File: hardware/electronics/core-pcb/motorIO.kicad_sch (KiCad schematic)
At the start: 3 parts, among them J5 1-84952-1, J6 1-84952-1, J7 1-84952-1

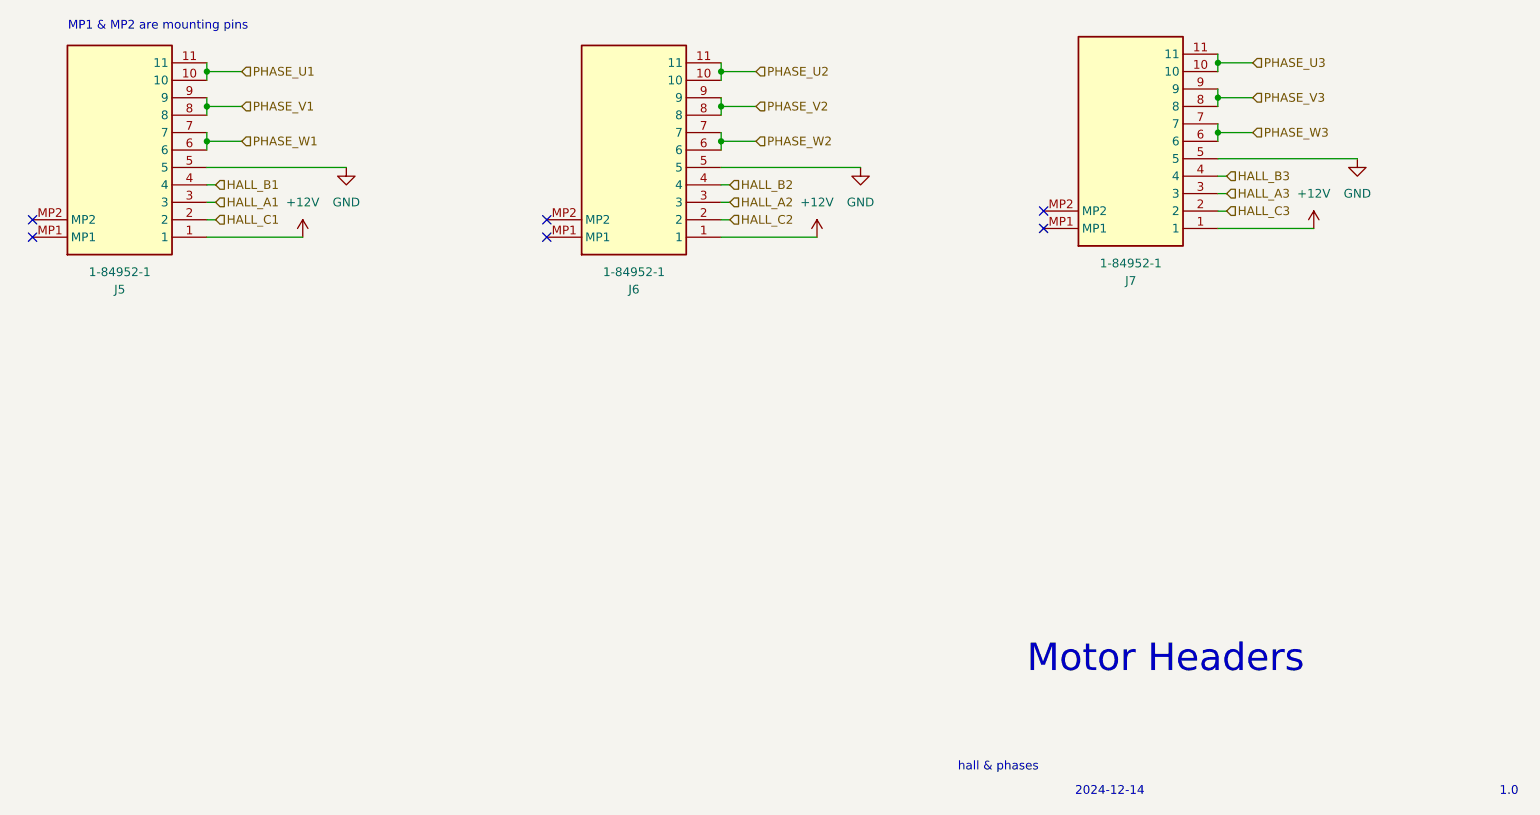
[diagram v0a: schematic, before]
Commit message: started work on pcbv2 work in progress
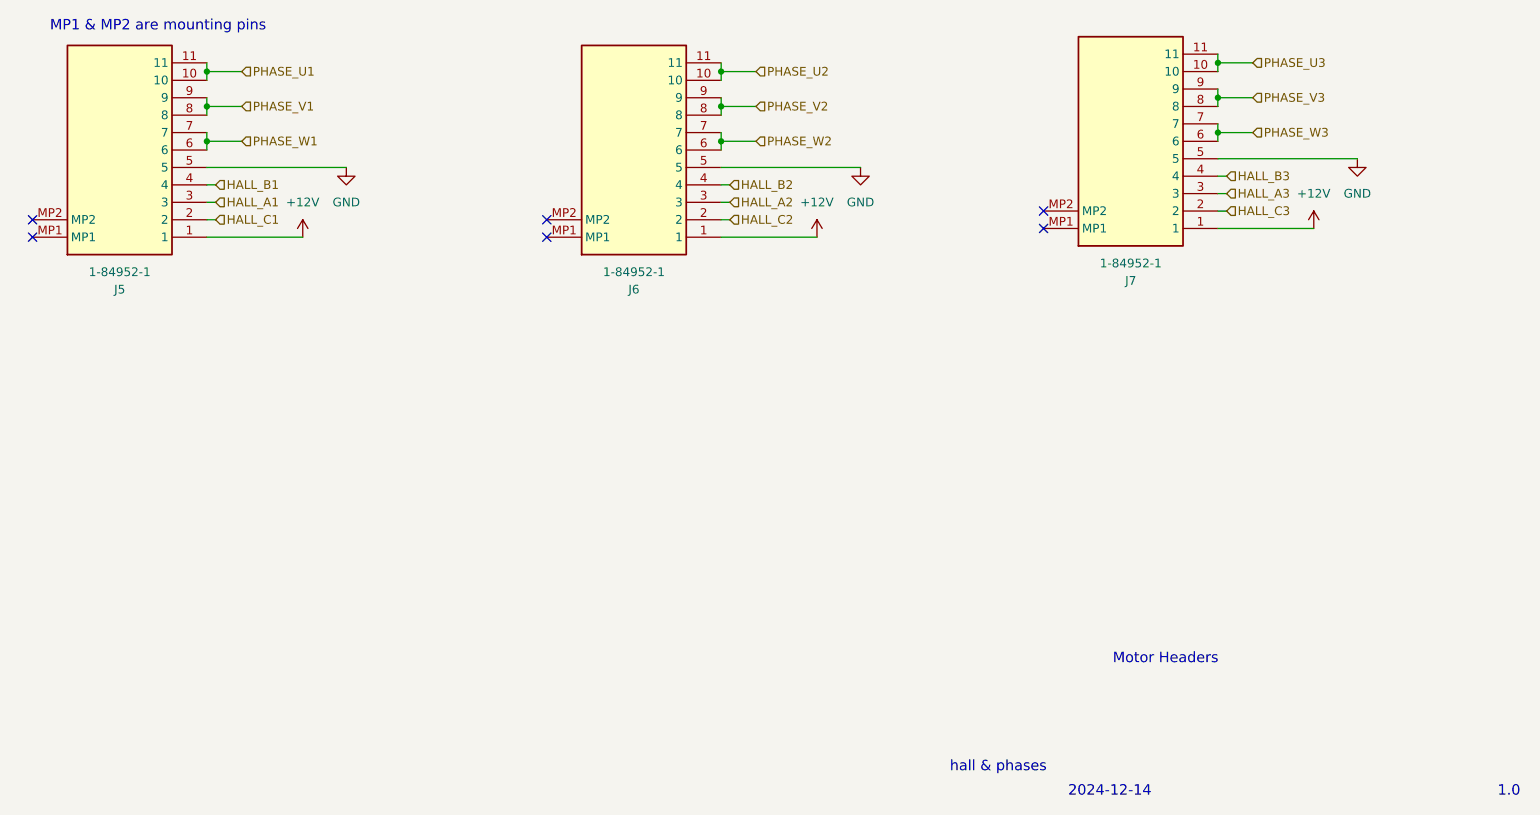
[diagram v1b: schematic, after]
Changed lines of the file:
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@@
 		(effects
 			(font
-				(size 1.27 1.27)
+				(face "Source Serif 4")
+				(size 1.524 1.524)
 			)
 		)
@@
 		(effects
 			(font
-				(size 1.27 1.27)
+				(face "Source Serif 4")
+				(size 1.524 1.524)
 			)
 		)
@@
 		(effects
 			(font
-				(size 4 4)
+				(face "Source Serif 4")
+				(size 1.524 1.524)
 			)
 		)
@@
 		(effects
 			(font
-				(size 1.27 1.27)
+				(face "Source Serif 4")
+				(size 1.524 1.524)
 			)
 		)
@@
 		(effects
 			(font
-				(size 1.27 1.27)
+				(face "Source Serif 4")
+				(size 1.524 1.524)
 			)
 		)
@@
 		)
 		(stroke
-			(width 0)
+			(width 0.1524)
 			(type default)
 		)
@@
 		)
 		(stroke
-			(width 0)
+			(width 0.1524)
 			(type default)
 		)
@@
 		)
 		(stroke
-			(width 0)
+			(width 0.1524)
 			(type default)
 		)
@@
 		)
 		(stroke
-			(width 0)
+			(width 0.1524)
 			(type default)
 		)
@@
 		)
 		(stroke
-			(width 0)
+			(width 0.1524)
 			(type default)
 		)
@@
 		)
 		(stroke
-			(width 0)
+			(width 0.1524)
 			(type default)
 		)
@@
 		)
 		(stroke
-			(width 0)
+			(width 0.1524)
 			(type default)
 		)
@@
 		)
 		(stroke
-			(width 0)
+			(width 0.1524)
 			(type default)
 		)
@@
 		)
 		(stroke
-			(width 0)
+			(width 0.1524)
 			(type default)
 		)
@@
 		)
 		(stroke
-			(width 0)
+			(width 0.1524)
 			(type default)
 		)
@@
 		)
 		(stroke
-			(width 0)
+			(width 0.1524)
 			(type default)
 		)
@@
 		)
 		(stroke
-			(width 0)
+			(width 0.1524)
 			(type default)
 		)
@@
 		)
 		(stroke
-			(width 0)
+			(width 0.1524)
 			(type default)
 		)
@@
 		)
 		(stroke
-			(width 0)
+			(width 0.1524)
 			(type default)
 		)
@@
 		)
 		(stroke
-			(width 0)
+			(width 0.1524)
 			(type default)
 		)
@@
 		)
 		(stroke
-			(width 0)
+			(width 0.1524)
 			(type default)
 		)
@@
 		)
 		(stroke
-			(width 0)
+			(width 0.1524)
 			(type default)
 		)
@@
 		)
 		(stroke
-			(width 0)
+			(width 0.1524)
 			(type default)
 		)
@@
 		)
 		(stroke
-			(width 0)
+			(width 0.1524)
 			(type default)
 		)
@@
 		)
 		(stroke
-			(width 0)
+			(width 0.1524)
 			(type default)
 		)
@@
 		)
 		(stroke
-			(width 0)
+			(width 0.1524)
 			(type default)
 		)
@@
 		)
 		(stroke
-			(width 0)
+			(width 0.1524)
 			(type default)
 		)
@@
 		)
 		(stroke
-			(width 0)
+			(width 0.1524)
 			(type default)
 		)
@@
 		)
 		(stroke
-			(width 0)
+			(width 0.1524)
 			(type default)
 		)
@@
 		)
 		(stroke
-			(width 0)
+			(width 0.1524)
 			(type default)
 		)
@@
 		)
 		(stroke
-			(width 0)
+			(width 0.1524)
 			(type default)
 		)
@@
 		)
 		(stroke
-			(width 0)
+			(width 0.1524)
 			(type default)
 		)
@@
 		)
 		(stroke
-			(width 0)
+			(width 0.1524)
 			(type default)
 		)
@@
 		)
 		(stroke
-			(width 0)
+			(width 0.1524)
 			(type default)
 		)
@@
 		)
 		(stroke
-			(width 0)
+			(width 0.1524)
 			(type default)
 		)
@@
 		)
 		(stroke
-			(width 0)
+			(width 0.1524)
 			(type default)
 		)
@@
 		)
 		(stroke
-			(width 0)
+			(width 0.1524)
 			(type default)
 		)
@@
 		)
 		(stroke
-			(width 0)
+			(width 0.1524)
 			(type default)
 		)
@@
 		)
 		(stroke
-			(width 0)
+			(width 0.1524)
 			(type default)
 		)
@@
 		)
 		(stroke
-			(width 0)
+			(width 0.1524)
 			(type default)
 		)
@@
 		)
 		(stroke
-			(width 0)
+			(width 0.1524)
 			(type default)
 		)
@@
 		)
 		(stroke
-			(width 0)
+			(width 0.1524)
 			(type default)
 		)
@@
 		)
 		(stroke
-			(width 0)
+			(width 0.1524)
 			(type default)
 		)
@@
 		)
 		(stroke
-			(width 0)
+			(width 0.1524)
 			(type default)
 		)
@@
 		)
 		(stroke
-			(width 0)
+			(width 0.1524)
 			(type default)
 		)
@@
 		)
 		(stroke
-			(width 0)
+			(width 0.1524)
 			(type default)
 		)
@@
 		)
 		(stroke
-			(width 0)
+			(width 0.1524)
 			(type default)
 		)
@@
 		(dnp no)
 		(fields_autoplaced yes)
-		(property "Reference" "#PWR0319"
+		(property "Reference" "#PWR0261"
 			(at 248.92 107.95 0)
 			(effects
@@
 			(project "motordriver"
 				(path "/c7634e88-16d1-45ec-9aac-9c841e03cf6d/5d8f5153-26a2-4903-a925-dc0c63f77bf7"
-					(reference "#PWR0319")
+					(reference "#PWR0261")
 					(unit 1)
 				)
@@
 		(dnp no)
 		(fields_autoplaced yes)
-		(property "Reference" "#PWR0314"
+		(property "Reference" "#PWR0256"
 			(at 95.25 116.84 0)
 			(effects
@@
 			(project "motordriver"
 				(path "/c7634e88-16d1-45ec-9aac-9c841e03cf6d/5d8f5153-26a2-4903-a925-dc0c63f77bf7"
-					(reference "#PWR0314")
+					(reference "#PWR0256")
 					(unit 1)
 				)
@@
 		(dnp no)
 		(fields_autoplaced yes)
-		(property "Reference" "#PWR0318"
+		(property "Reference" "#PWR0260"
 			(at 242.57 115.57 0)
 			(effects
@@
 			(project "motordriver"
 				(path "/c7634e88-16d1-45ec-9aac-9c841e03cf6d/5d8f5153-26a2-4903-a925-dc0c63f77bf7"
-					(reference "#PWR0318")
+					(reference "#PWR0260")
 					(unit 1)
 				)
@@
 		(dnp no)
 		(fields_autoplaced yes)
-		(property "Reference" "#PWR0315"
+		(property "Reference" "#PWR0257"
 			(at 101.6 109.22 0)
 			(effects
@@
 			(project "motordriver"
 				(path "/c7634e88-16d1-45ec-9aac-9c841e03cf6d/5d8f5153-26a2-4903-a925-dc0c63f77bf7"
-					(reference "#PWR0315")
+					(reference "#PWR0257")
 					(unit 1)
 				)
@@
 		(dnp no)
 		(fields_autoplaced yes)
-		(property "Reference" "#PWR0317"
+		(property "Reference" "#PWR0259"
 			(at 176.53 109.22 0)
 			(effects
@@
 			(project "motordriver"
 				(path "/c7634e88-16d1-45ec-9aac-9c841e03cf6d/5d8f5153-26a2-4903-a925-dc0c63f77bf7"
-					(reference "#PWR0317")
+					(reference "#PWR0259")
 					(unit 1)
 				)
@@
 		(dnp no)
 		(fields_autoplaced yes)
-		(property "Reference" "#PWR0316"
+		(property "Reference" "#PWR0258"
 			(at 170.18 116.84 0)
 			(effects
@@
 			(project "motordriver"
 				(path "/c7634e88-16d1-45ec-9aac-9c841e03cf6d/5d8f5153-26a2-4903-a925-dc0c63f77bf7"
-					(reference "#PWR0316")
+					(reference "#PWR0258")
 					(unit 1)
 				)
